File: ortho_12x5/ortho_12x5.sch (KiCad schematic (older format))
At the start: 120 parts, among them SW1 SW_SPST, SW10 SW_SPST, SW11 SW_SPST, SW12 SW_SPST, SW13 SW_SPST, SW14 SW_SPST, SW15 SW_SPST, SW16 SW_SPST, SW17 SW_SPST, SW18 SW_SPST, SW19 SW_SPST, SW2 SW_SPST, SW20 SW_SPST, SW21 SW_SPST, SW22 SW_SPST, SW23 SW_SPST, SW24 SW_SPST, SW25 SW_SPST, SW26 SW_SPST, SW27 SW_SPST, SW28 SW_SPST, SW29 SW_SPST, SW3 SW_SPST, SW30 SW_SPST, SW31 SW_SPST, SW32 SW_SPST, SW33 SW_SPST, SW34 SW_SPST, SW35 SW_SPST, SW36 SW_SPST, SW37 SW_SPST, SW38 SW_SPST, SW39 SW_SPST, SW4 SW_SPST, SW40 SW_SPST, SW41 SW_SPST, SW42 SW_SPST, SW43 SW_SPST, SW44 SW_SPST, SW45 SW_SPST, SW46 SW_SPST, SW47 SW_SPST, SW48 SW_SPST, SW49 SW_SPST, SW5 SW_SPST, SW50 SW_SPST, SW51 SW_SPST, SW52 SW_SPST, SW53 SW_SPST, SW54 SW_SPST, SW55 SW_SPST, SW56 SW_SPST, SW57 SW_SPST, SW58 SW_SPST, SW59 SW_SPST, SW6 SW_SPST, SW60 SW_SPST, SW7 SW_SPST, SW8 SW_SPST, SW9 SW_SPST

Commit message: Start layout
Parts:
- D1, D10, D11, D12, D13, D14, D15, D16, D17, D18, D19, D2, D20, D21, D22, D23, D24, D25, D26, D27, D28, D29, D3, D30, D31, D32, D33, D34, D35, D36, D37, D38, D39, D4, D40, D41, D42, D43, D44, D45, D46, D47, D48, D49, D5, D50, D51, D52, D53, D54, D55, D56, D57, D58, D59, D6, D60, D7, D8, D9: footprint (none) -> Diode_THT:D_DO-34_SOD68_P7.62mm_Horizontal

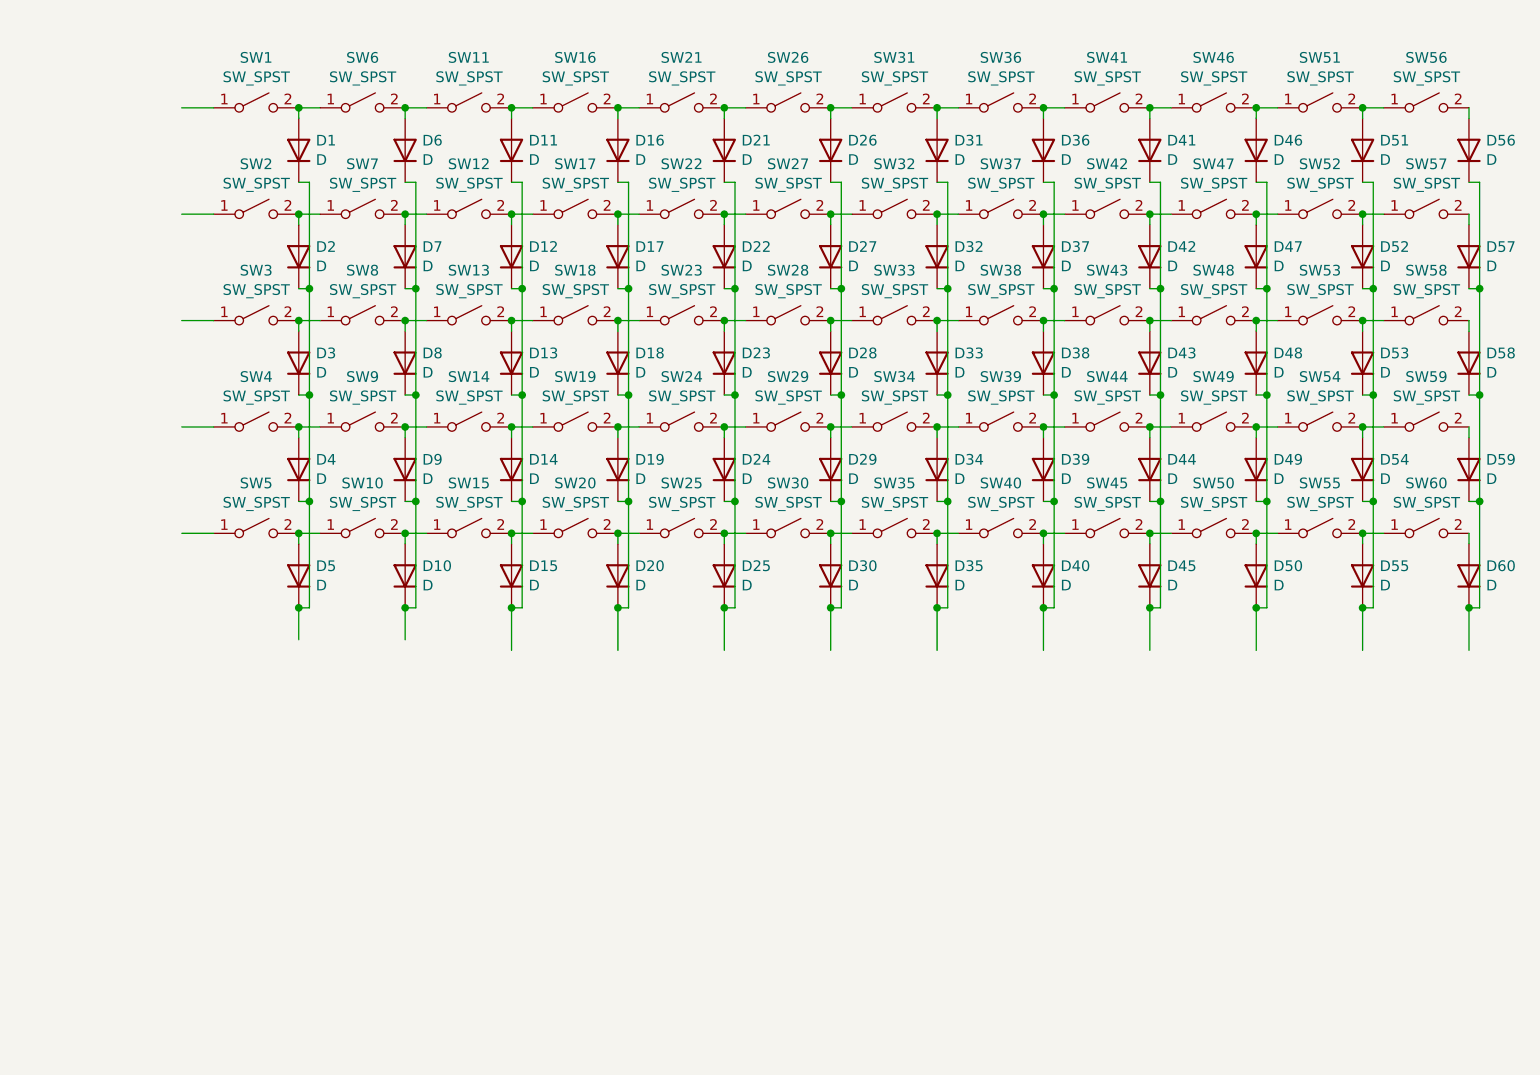
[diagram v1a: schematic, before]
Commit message: Redo schematic
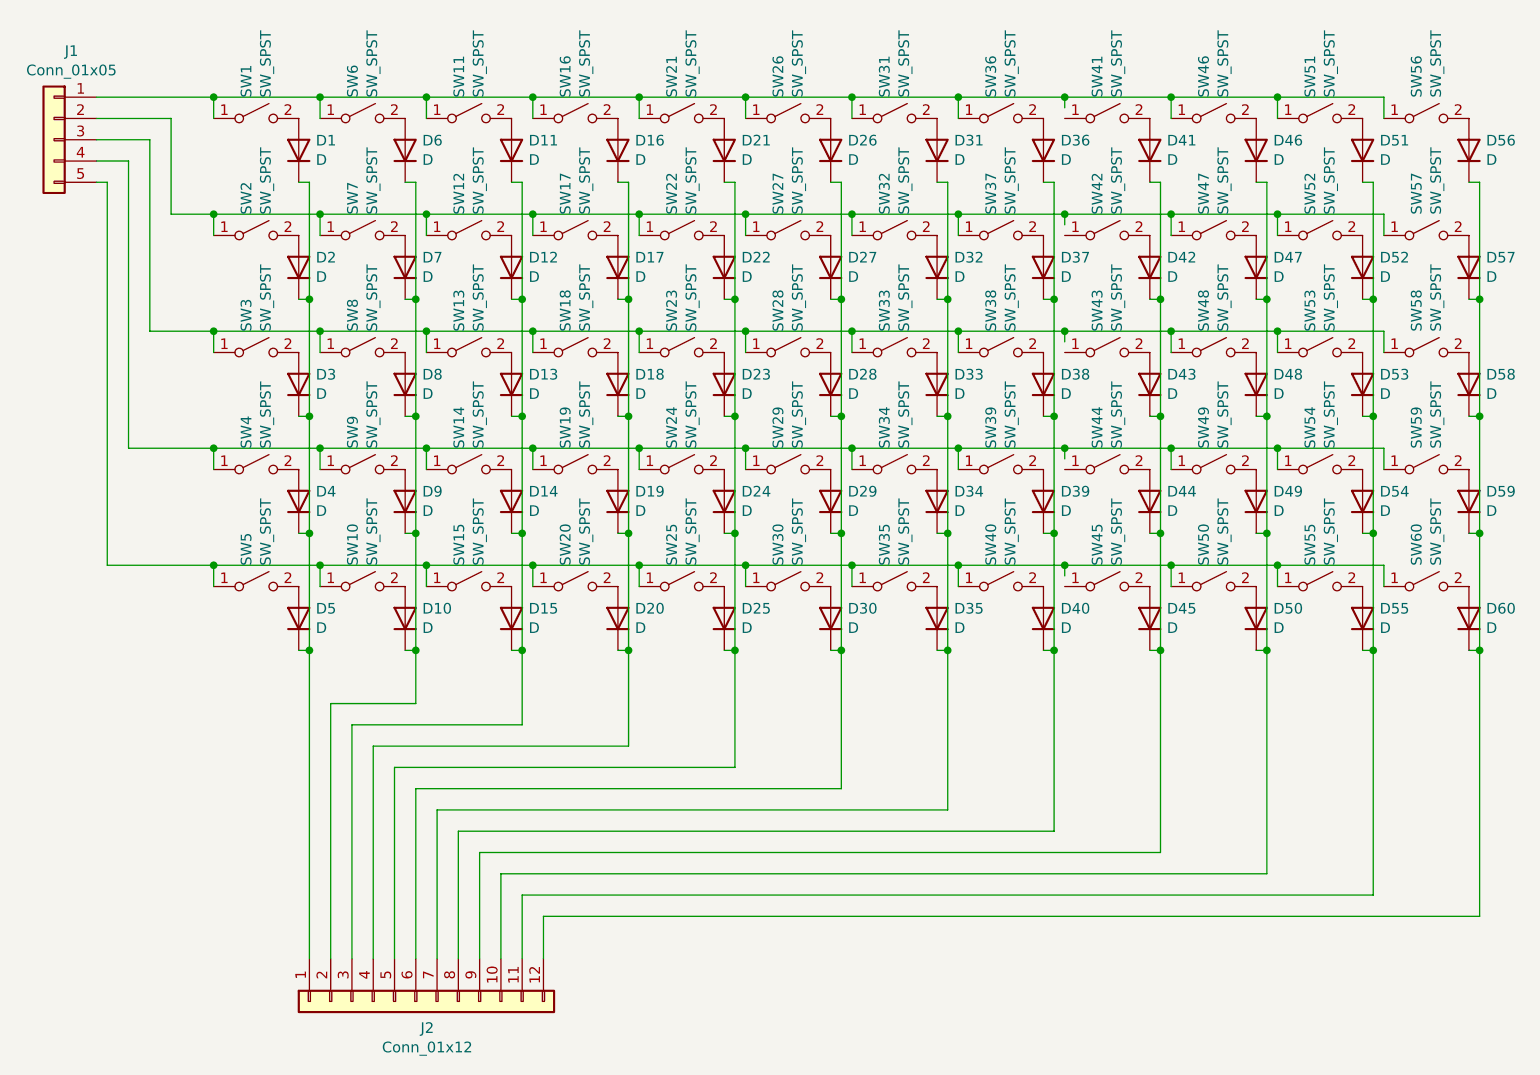
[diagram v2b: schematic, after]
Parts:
- added J1: Conn_01x05, Connector_PinSocket_2.54mm:PinSocket_1x05_P2.54mm_Horizontal, symbol Connector_Generic:Conn_01x05
- added J2: Conn_01x12, Connector_PinHeader_2.54mm:PinHeader_1x12_P2.54mm_Horizontal, symbol Connector_Generic:Conn_01x12
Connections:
- wire segments 240 -> 270
